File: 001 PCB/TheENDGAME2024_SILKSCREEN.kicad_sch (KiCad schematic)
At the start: 78 parts, among them J1 B+, J2 B-, SW1 SW_SPDT, SW10 SW_Push, SW11 SW_Push, SW12 SW_Push, SW13 SW_Push, SW14 SW_Push, SW15 SW_Push, SW16 SW_Push, SW17 SW_Push, SW18 SW_Push, SW19 SW_Push, SW2 SW_Push, SW20 SW_Push, SW21 SW_Push, SW22 SW_Push, SW23 SW_Push, SW24 SW_Push, SW25 SW_Push, SW26 SW_Push, SW27 SW_Push, SW28 SW_Push, SW29 SW_Push, SW3 SW_Push, SW30 SW_Push, SW31 SW_Push, SW32 SW_Push, SW33 SW_Push, SW34 SW_Push, SW35 SW_Push, SW36 SW_Push, SW37 SW_Push, SW38 SW_Push, SW4 SW_Push, SW5 SW_Push, SW6 SW_Push, SW7 SW_Push, SW8 SW_Push, SW9 SW_Push, U1 SuperMini nRF52840, U2 RP2040-Zero_stolen_from_Purox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

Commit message: 3d models
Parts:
- D10, D11, D12, D13, D14, D15, D17, D18, D19, D20, D22, D23, D24, D25, D26, D27, D28, D29, D32, D33, D34, D35, D36, D37, D38, D39, D40, D41, D44, D45, D46, D47, D5, D6, D7, D8: footprint TheEndgame2024:Diode_SOD123 filets triangle -> TheEndgame2024:Diode_SOD123_3D
- SW10, SW11, SW12, SW13, SW14, SW15, SW16, SW17, SW18, SW19, SW2, SW20, SW21, SW22, SW23, SW24, SW25, SW26, SW27, SW28, SW29, SW3, SW30, SW31, SW32, SW33, SW34, SW35, SW36, SW37, SW4, SW5, SW6, SW7, SW8, SW9: footprint Cherry_ULP:Cherry_ULP_TH_CUT -> TheEndgame2024:Cherry_ULP_TH_CUT_3D
- U1: footprint PCM_marbastlib-xp-promicroish:SuperMini_nRF52840_AH_USBup -> TheEndgame2024:SuperMini_nRF52840_AH_USBup_3D

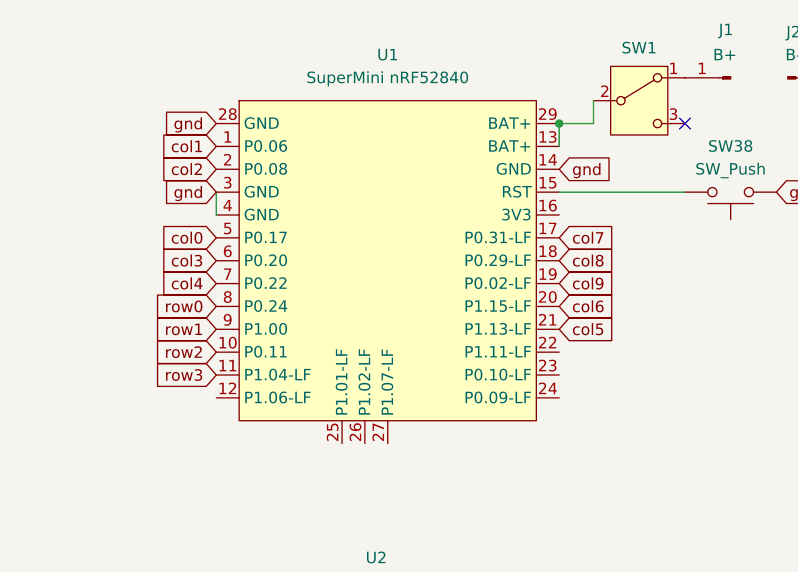
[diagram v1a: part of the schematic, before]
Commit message: moved everything to the top
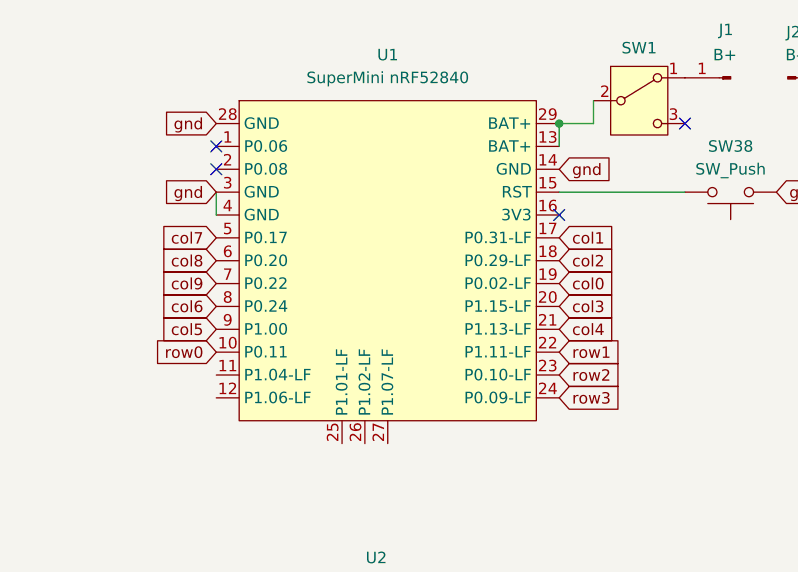
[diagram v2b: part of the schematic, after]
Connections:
- net col0: now also U1.19 (P0.02-LF); no longer U1.5 (P0.17)
- net col1: now also U1.17 (P0.31-LF); no longer U1.1 (P0.06)
- net col2: now also U1.18 (P0.29-LF); no longer U1.2 (P0.08)
- net col3: now also U1.20 (P1.15-LF); no longer U1.6 (P0.20)
- net col4: now also U1.21 (P1.13-LF); no longer U1.7 (P0.22)
- net col5: now also U1.9 (P1.00); no longer U1.21 (P1.13-LF)
- net col6: now also U1.8 (P0.24); no longer U1.20 (P1.15-LF)
- net col7: now also U1.5 (P0.17); no longer U1.17 (P0.31-LF)
- net col8: now also U1.6 (P0.20); no longer U1.18 (P0.29-LF)
- net col9: now also U1.7 (P0.22); no longer U1.19 (P0.02-LF)
- net row0: now also U1.10 (P0.11); no longer U1.8 (P0.24)
- net row1: now also U1.22 (P1.11-LF); no longer U1.9 (P1.00)
- net row2: now also U1.23 (P0.10-LF); no longer U1.10 (P0.11)
- net row3: now also U1.24 (P0.09-LF); no longer U1.11 (P1.04-LF)
- no-connect marks 8 -> 11
